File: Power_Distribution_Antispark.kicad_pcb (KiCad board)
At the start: 2 copper layers, 131 parts, among them J1 STM Signal Conn, J10 CSense12V_2 Conn, J11 CSense12V_3 Conn, J2 +48V Battery Conn, J3 Motor Conn, J4 CSense3V3STM Conn, J5 CSense3V3_2 Conn, J6 CSense5V_1 Conn, J7 CSense5V_2 Conn, J8 CSense5V_3 Conn, J9 CSense12V_1 Conn, Q1 BUK9M42-60EX, Q2 G20P06K, Q3 BUK9M42-60EX, Q4 G20P06K, U1 TLV74033PDBVR, U10 INA181A3IDBVR, U11 INA181A3IDBVR, U12 INA181A3IDBVR, U13 INA181A3IDBVR, U14 INA181A3IDBVR, U2 74LVC1G14GW_125, U3 TPP60308-ES1R-S, U4 TPP60308-ES1R-S, U5 LM331AU-S5TR, U6 INA181A3IDBVR, U7 INA181A3IDBVR, U8 INA181A3IDBVR, U9 INA181A3IDBVR

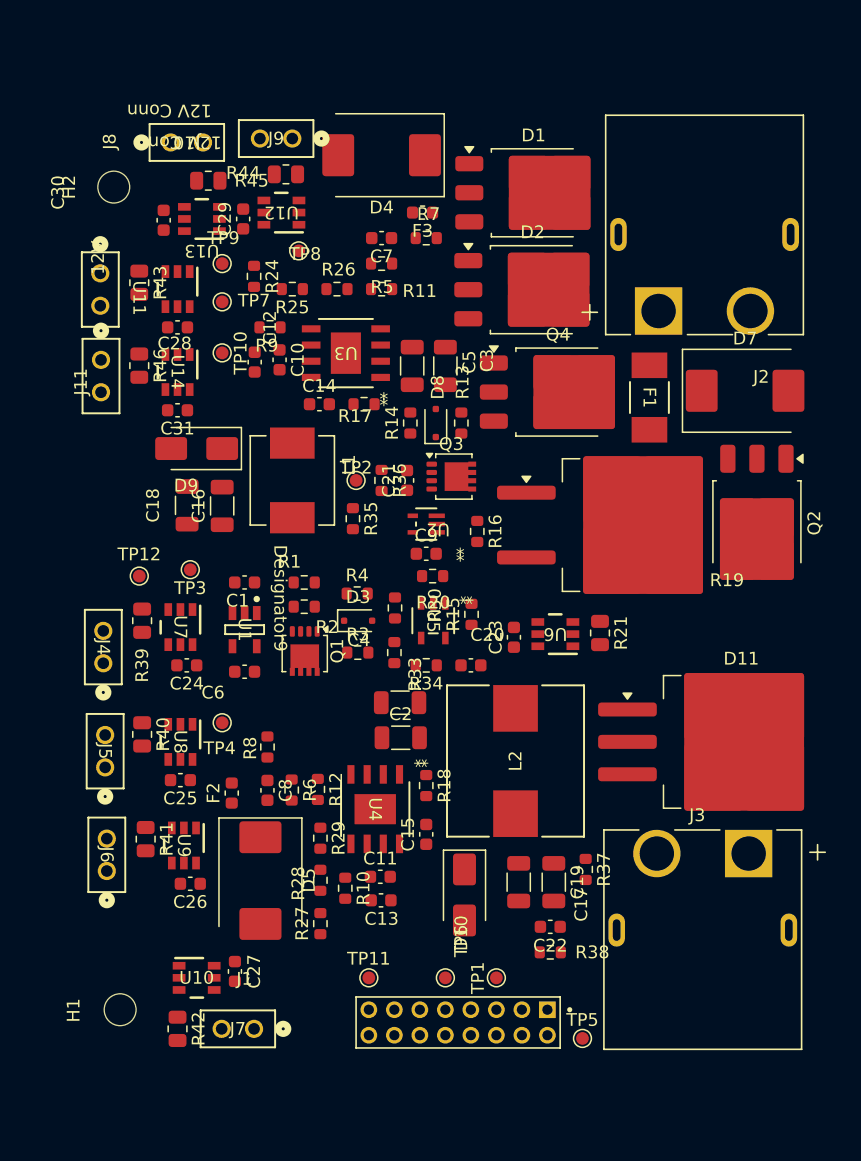
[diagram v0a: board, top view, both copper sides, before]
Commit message: layout2
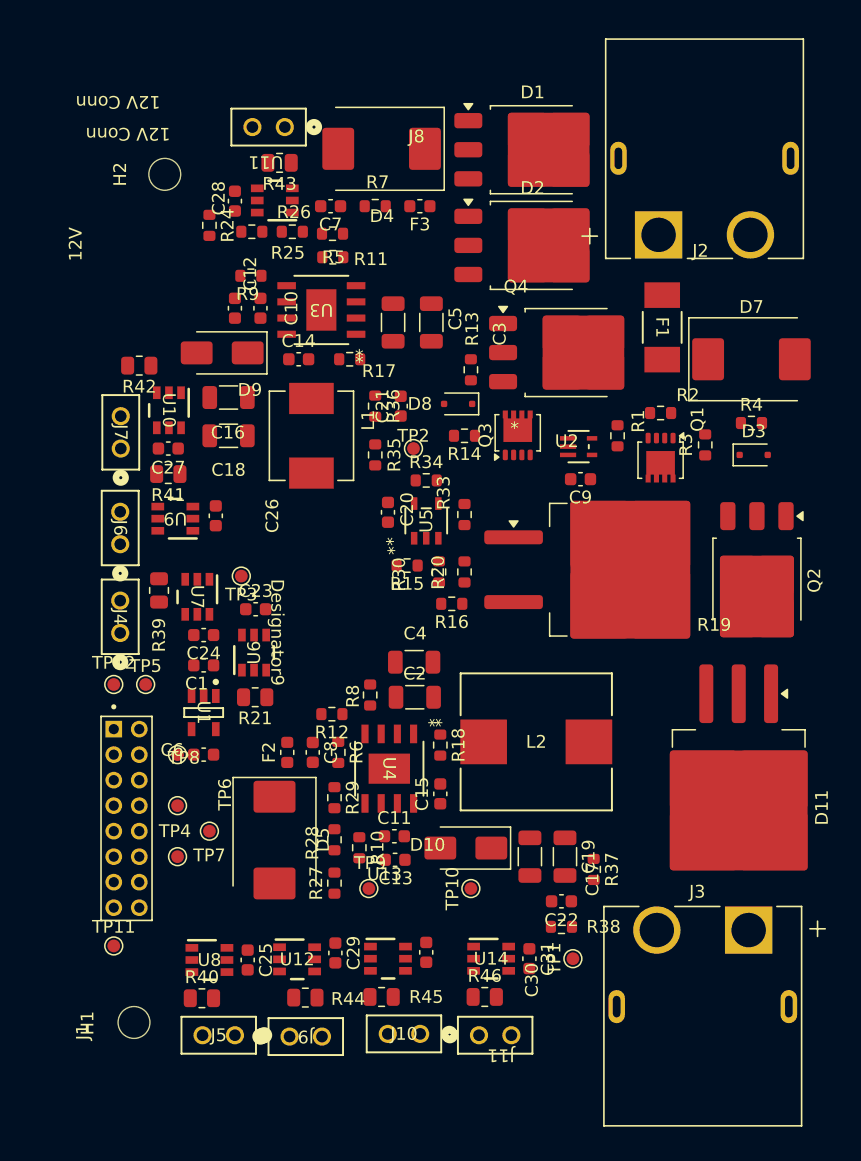
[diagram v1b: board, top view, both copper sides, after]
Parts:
- moved J10 72.6 mm to (190.5, 122.9), turned to 0 degrees
- moved J9 70.4 mm to (180.3, 123.1), turned to 180 degrees
- moved R45 65.4 mm to (187.5, 120.0)
- moved R44 64.6 mm to (181.5, 120.1), turned to 0 degrees
- moved C30 61.0 mm to (191.0, 116.5), turned to -90 degrees
- moved J11 60.7 mm to (195.1, 123.0), turned to 180 degrees
- moved U13 59.8 mm to (188.0, 117.0), turned to 0 degrees
- moved U12 58.6 mm to (180.9, 117.1), turned to 0 degrees
- moved C29 58.0 mm to (183.9, 116.6), turned to -90 degrees
- moved R46 56.4 mm to (195.6, 120.0), turned to 0 degrees
- moved U14 52.2 mm to (196.1, 117.0), turned to 0 degrees
- moved R42 52.1 mm to (168.5, 70.5), turned to 180 degrees
- moved C31 51.1 mm to (199.1, 117.0), turned to -90 degrees
- moved TP9 50.3 mm to (186.5, 111.5)
- moved J7 46.7 mm to (167.0, 77.0), turned to -90 degrees
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
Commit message: Add files via upload
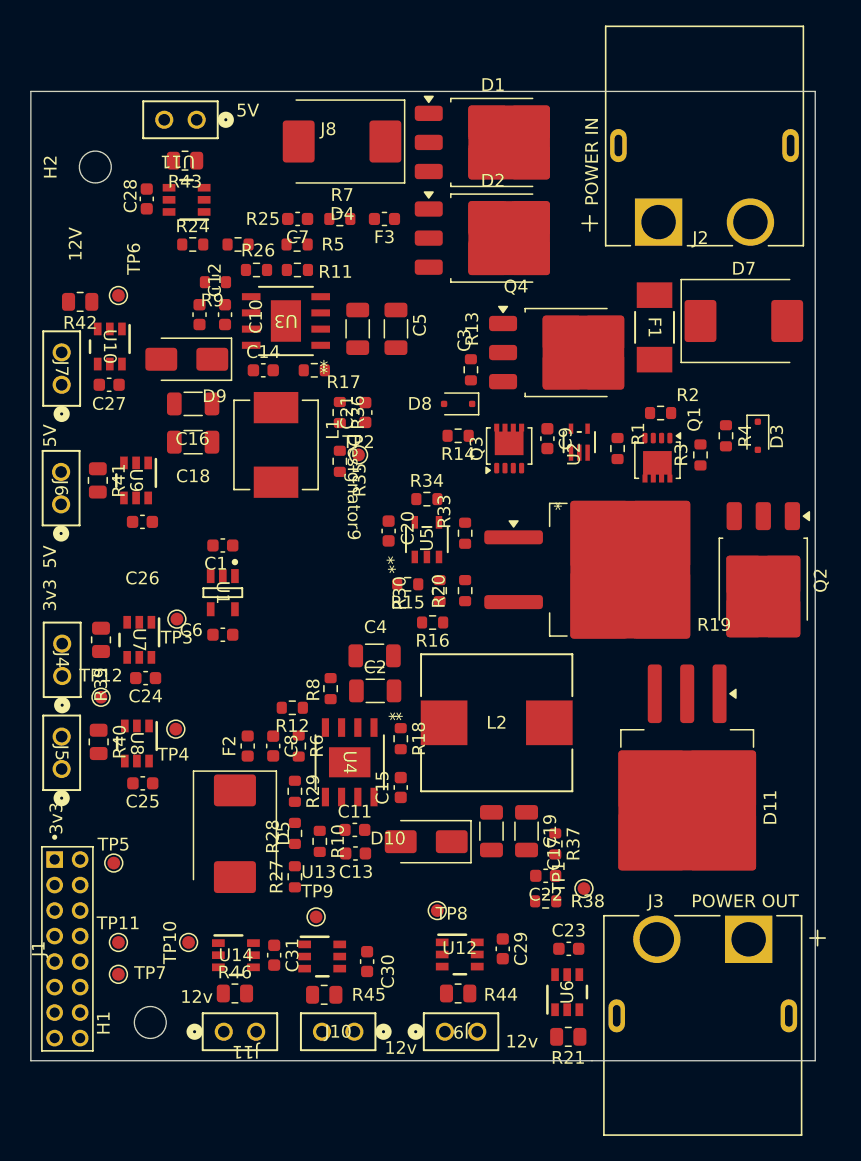
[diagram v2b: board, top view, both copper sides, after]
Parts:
- moved TP6 42.6 mm to (166.9, 65.0)
- moved R21 36.2 mm to (202.1, 123.1)
- moved U6 36.2 mm to (202.1, 119.6)
- moved C23 36.2 mm to (202.2, 116.2)
- moved J5 24.9 mm to (162.4, 102.1), turned to -90 degrees
- moved TP8 23.8 mm to (191.9, 113.2)
- moved TP10 22.5 mm to (172.4, 115.7)
- moved R40 21.7 mm to (165.3, 100.0), turned to -90 degrees
- moved C31 20.0 mm to (179.1, 116.7)
- moved J11 20.0 mm to (175.1, 122.7)
- moved U14 20.0 mm to (176.1, 116.7)
- moved R46 19.6 mm to (176.0, 119.7)
- moved U8 17.9 mm to (168.3, 100.1), turned to -90 degrees
- moved C25 16.1 mm to (168.8, 103.2), turned to 180 degrees
- moved TP5 14.2 mm to (166.5, 109.5)
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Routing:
- added copper zone on In1.Cu, net GND
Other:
- board outline added: 61.5 x 76 mm
- copper layers 2 -> 4
- board text added: "12v"
- board text added: "3v3"
- board text added: "5V"
- board text added: "POWER IN"
- board text added: "POWER OUT"
- board text removed: "12V Conn"
